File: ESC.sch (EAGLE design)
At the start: 50 parts, among them U1 AMS1117-3.3

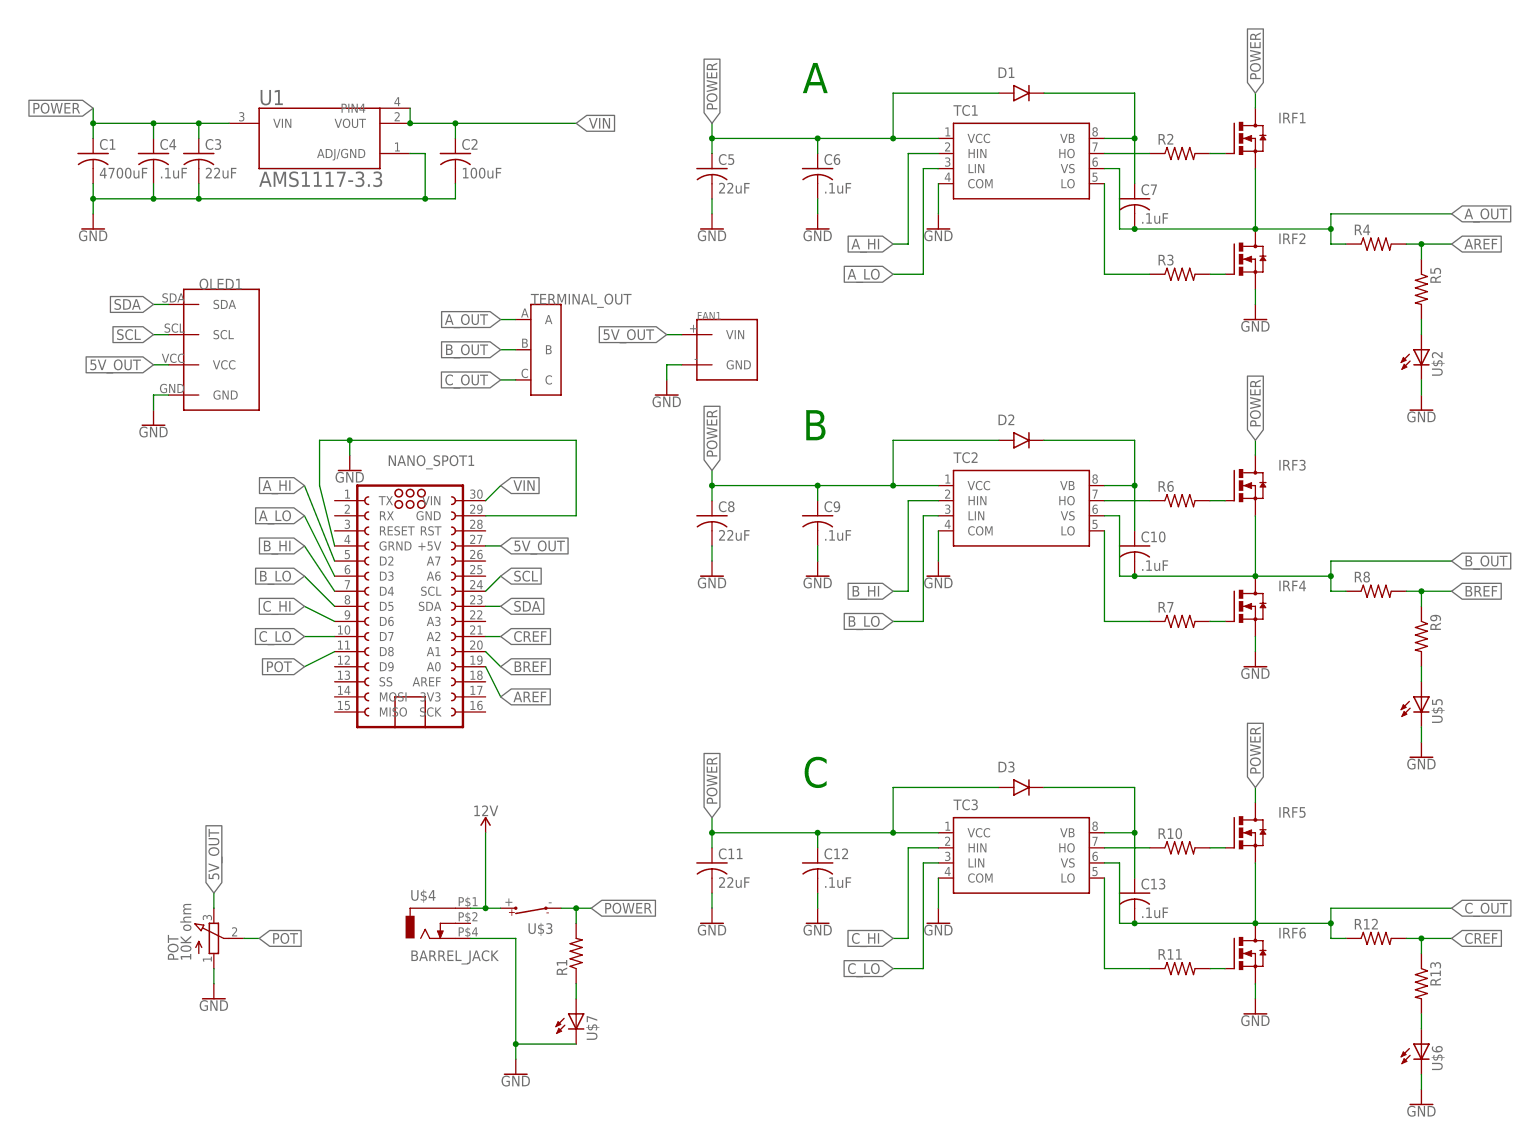
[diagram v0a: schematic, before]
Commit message: late changes 10052018
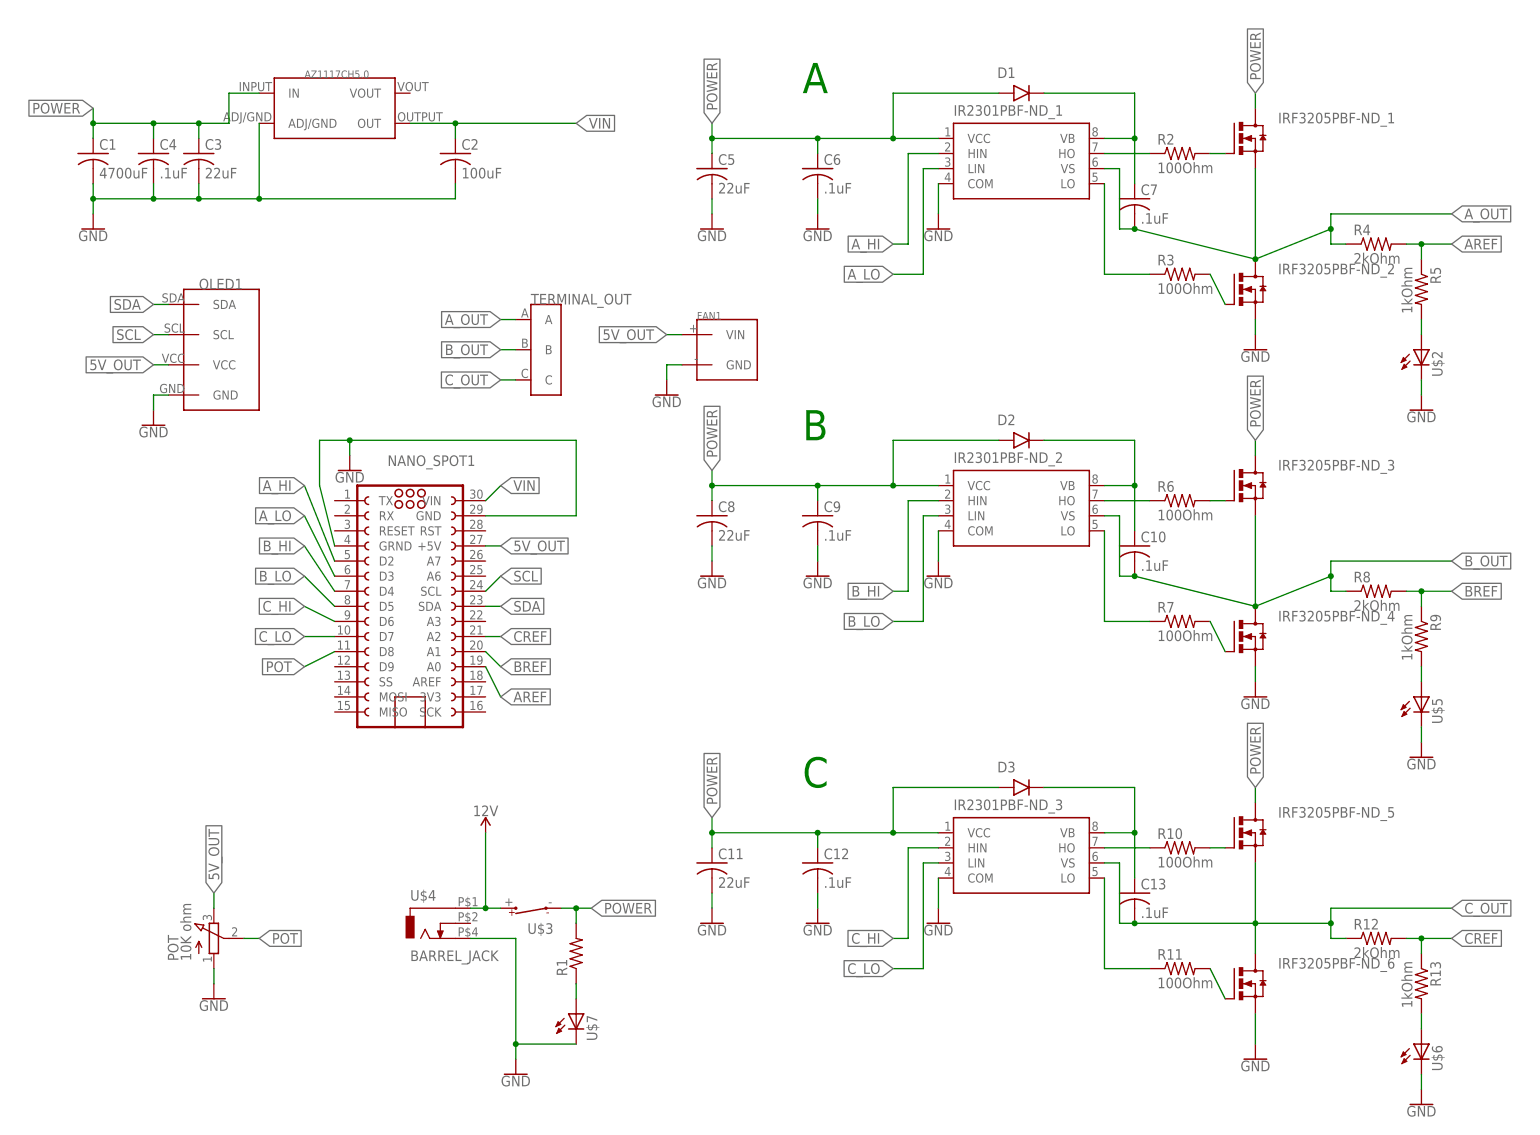
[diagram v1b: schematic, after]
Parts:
- removed IRF2, IRF4, IRF6: (no value), TRANS_IRF3205SPBF:IRF3205
- removed U1: AMS1117-3.3, AMS1117-3.3:AMS1117-3.3
- added AZ1117CH5.0: AZ1117CH, TRANS_IRF3205SPBF:AZ1117CH
- added IRF3205PBF-ND_2, IRF3205PBF-ND_4, IRF3205PBF-ND_6: (no value), TRANS_IRF3205SPBF:IRF3205
- R10, R11, R2, R3, R6, R7: value (none) -> 100Ohm
- R12, R4, R8: value (none) -> 2kOhm
- R13, R5, R9: value (none) -> 1kOhm
- renumbered IRF1 to IRF3205PBF-ND_1, IRF3 to IRF3205PBF-ND_3, IRF5 to IRF3205PBF-ND_5, TC1 to IR2301PBF-ND_1, TC2 to IR2301PBF-ND_2, TC3 to IR2301PBF-ND_3
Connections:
- net A_OUT: now also IRF3205PBF-ND_2.D; no longer IRF2.D
- net B_OUT: now also IRF3205PBF-ND_4.D; no longer IRF4.D
- net C_OUT: now also IRF3205PBF-ND_6.D; no longer IRF6.D
- net GND: now also AZ1117CH5.0.ADJ/GND, IRF3205PBF-ND_2.S, IRF3205PBF-ND_4.S, IRF3205PBF-ND_6.S; no longer IRF2.S, IRF4.S, IRF6.S, U1.ADJ/GND
- net N$1: now also IRF3205PBF-ND_2.G; no longer IRF2.G
- net N$14: now also IRF3205PBF-ND_4.G; no longer IRF4.G
- net N$24: now also IRF3205PBF-ND_6.G; no longer IRF6.G
- net POWER: now also AZ1117CH5.0.IN; no longer U1.VIN
- net VIN: now also AZ1117CH5.0.OUT; no longer U1.PIN4, U1.VOUT
